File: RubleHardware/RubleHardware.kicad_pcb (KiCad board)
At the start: 4 copper layers, 56.5 x 75.4 mm, 46 parts, among them IC1 LTC3780EUH#PBF, J1_IN1 Conn_01x08_Male, J2_OUT1 Conn_01x08_Male

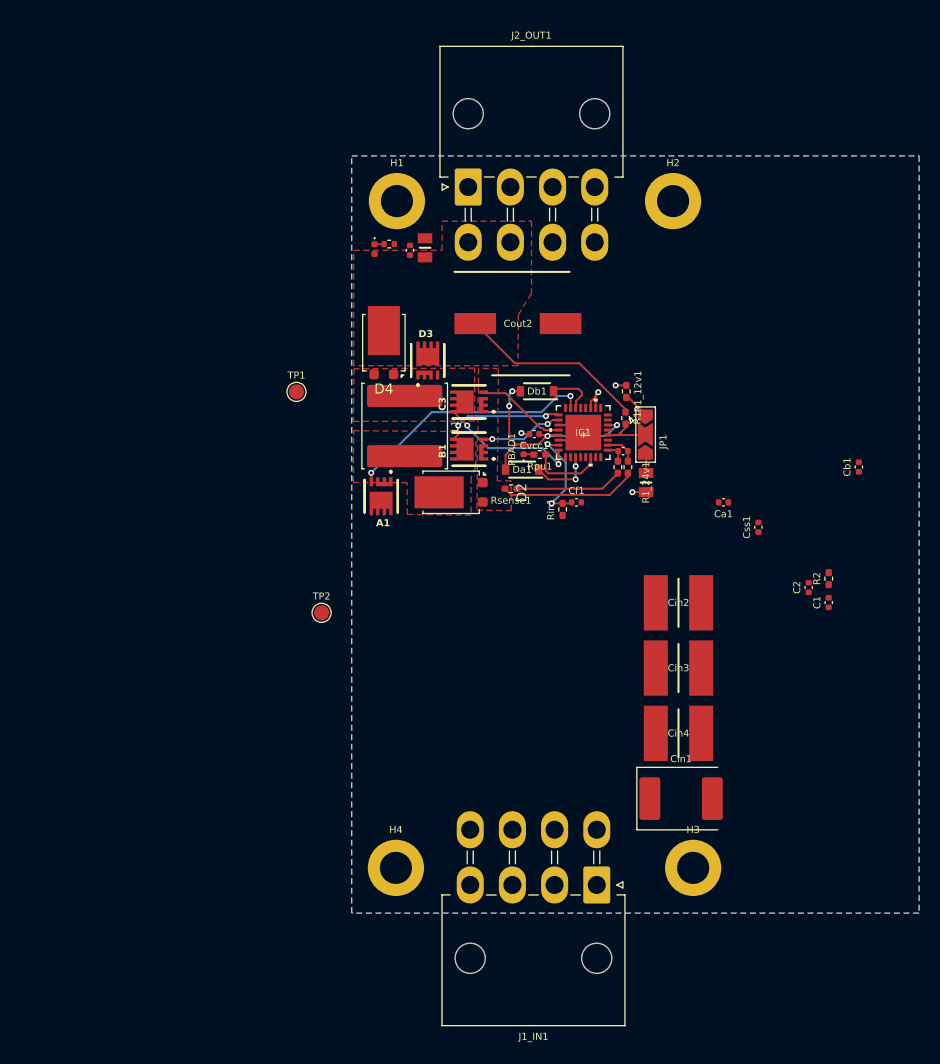
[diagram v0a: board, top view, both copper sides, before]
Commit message: feat: First board revision
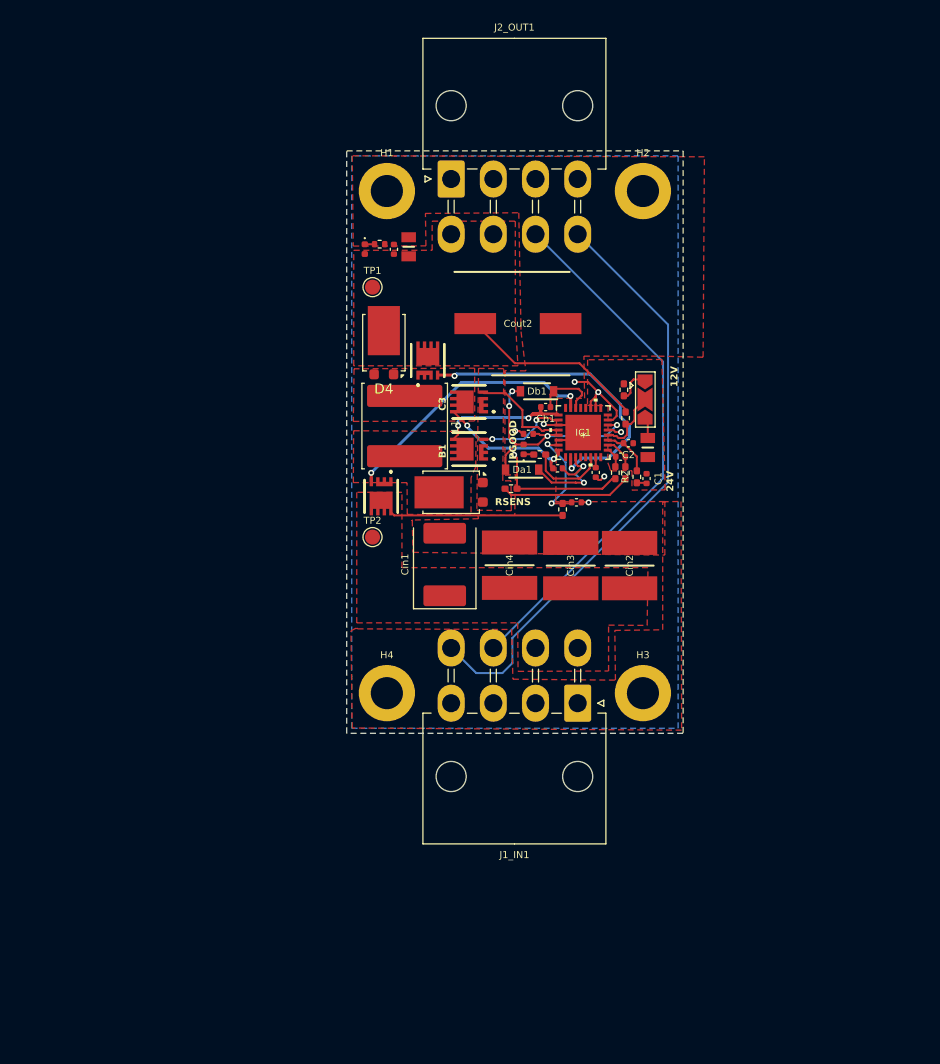
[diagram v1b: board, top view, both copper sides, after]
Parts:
- moved Cin1 33.1 mm to (168.3, 100.2), turned to 90 degrees
- moved Cb1 31.8 mm to (178.3, 84.5), turned to 180 degrees
- moved Cin4 23.7 mm to (174.7, 100.3), turned to -90 degrees
- moved C2 23.0 mm to (186.6, 88.1), turned to 180 degrees
- moved C1 21.9 mm to (188.4, 91.6), turned to -90 degrees
- moved R2 21.6 mm to (187.4, 91.5)
- moved J1_IN1 18.2 mm to (181.5, 114.0)
- moved H3 18.1 mm to (188.0, 113.0)
- moved H4 17.4 mm to (162.5, 113.0)
- moved Css1 17.1 mm to (183.3, 91.0)
- moved Ca1 16.9 mm to (179.5, 90.6)
- moved Cin3 14.8 mm to (180.8, 100.3), turned to -90 degrees
- moved TP1 12.9 mm to (161.1, 72.6)
- moved TP2 9.09 mm to (161.1, 97.5)
- moved Cin2 6.12 mm to (186.7, 100.3), turned to -90 degrees
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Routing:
- net /CAN+: track 0.00 -> 60.4 mm
- net /CAN-: track 0.00 -> 53.5 mm
- net /TG1: track 0.00 -> 31.4 mm, vias 0 -> 2
- net /ICVIN: track 0.00 -> 17.2 mm
- net GND: track 22.5 -> 34.9 mm, vias 4 -> 8
- net Net-(Da1-K): track 6.29 -> 11.8 mm
- net Net-(IC1-ITH): track 0.00 -> 5.00 mm
- net /SW2: track 12.1 -> 14.1 mm
- net Net-(Db1-K): track 4.61 -> 6.31 mm
- net /TG2: track 25.1 -> 26.2 mm
- net /BG1: track 8.99 -> 10.1 mm
- net Net-(IC1-SS): track 0.00 -> 1.07 mm
- net Net-(C1-Pad2): track 0.00 -> 0.99 mm
- net Net-(JP1-A): track 2.61 -> 3.40 mm
- net Net-(IC1-PGOOD): track 7.25 -> 7.94 mm
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- added copper zone on In2.Cu, net +3V3
- added copper zone on F.Cu, net /ICVIN
- added copper zone on B.Cu, net GND
- added copper zone on F.Cu, net GND
- added copper zone on In1.Cu, net GND
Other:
- board size 56.5 x 75.4 mm -> 33.5 x 58 mm
- board text added: "12V"
- board text added: "24V"
- board text added: "PGOOD"
- board text added: "RSENS"

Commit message: feat: Board V2
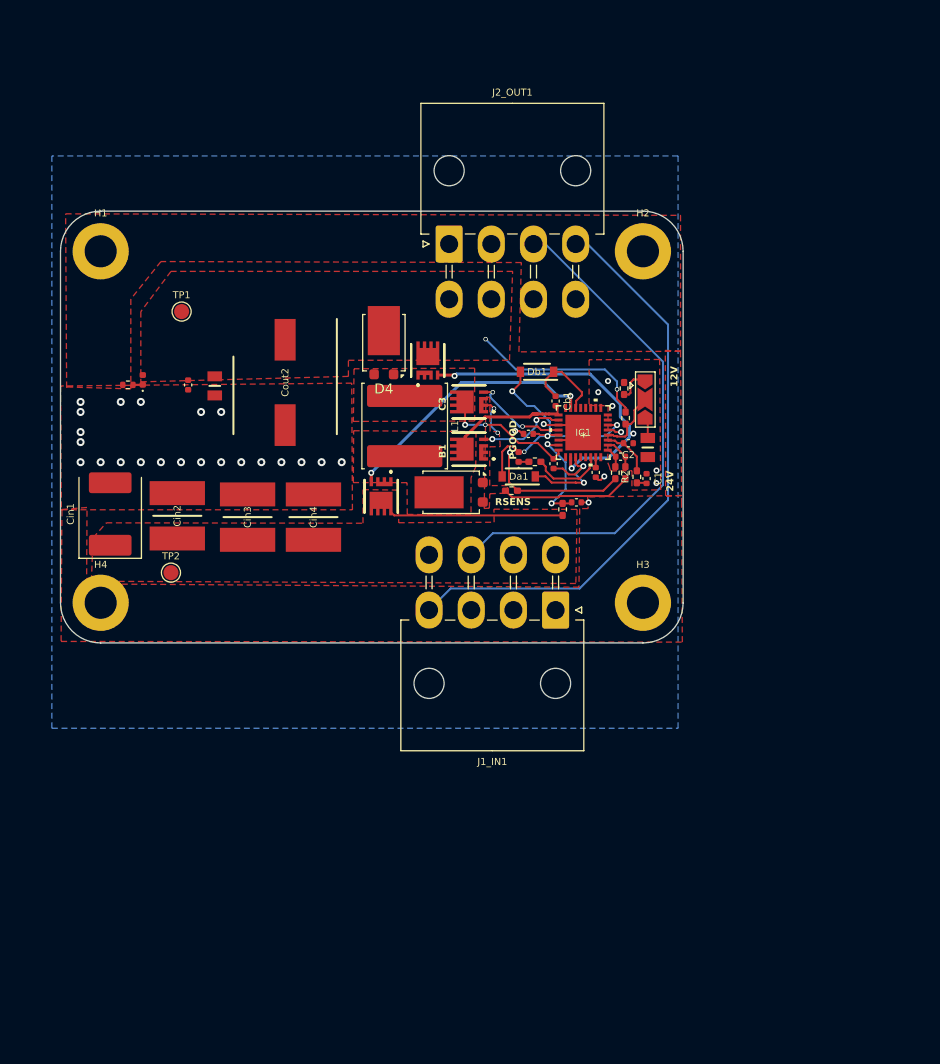
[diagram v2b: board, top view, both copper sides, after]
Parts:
- moved Cin2 45.3 mm to (141.6, 95.3)
- moved Cin1 33.7 mm to (134.9, 95.2)
- moved Cin3 32.5 mm to (148.6, 95.5)
- moved H4 29.9 mm to (134.0, 104.0)
- moved H1 29.1 mm to (134.0, 69.0)
- moved R3 28.7 mm to (136.7, 82.3), turned to 180 degrees
- moved D1 25.7 mm to (138.2, 81.8), turned to 90 degrees
- moved Cout1 24.5 mm to (142.7, 82.3), turned to -90 degrees
- moved Cout2 23.9 mm to (152.4, 82.1), turned to -90 degrees
- moved Cout3 23.8 mm to (145.4, 82.4), turned to -90 degrees
- moved TP2 20.4 mm to (141.0, 101.0)
- moved Cin4 20.1 mm to (155.2, 95.5)
- moved TP1 19.2 mm to (142.1, 75.0)
- moved J1_IN1 9.53 mm to (179.3, 104.7)
- moved H3 9.00 mm to (188.0, 104.0)
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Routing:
- net +3V3: track 0.00 -> 58.5 mm
- net /CAN-: track 53.5 -> 91.0 mm
- net /CAN+: track 60.4 -> 31.5 mm
- net GND: track 34.9 -> 25.7 mm, vias 8 -> 34
- net /INTVCC: track 26.1 -> 30.0 mm
- net /SENS-: track 13.4 -> 17.2 mm, vias 0 -> 2
- net Net-(Db1-K): track 6.31 -> 8.37 mm
- net /SW2: track 14.1 -> 13.1 mm, vias 2 -> 0
- net Net-(Da1-K): track 11.8 -> 12.5 mm
- net /ICVOUT: track 18.8 -> 18.2 mm, vias 0 -> 2
- net Net-(IC1-PGOOD): track 7.94 -> 7.42 mm
- net /BG1: track 10.1 -> 9.68 mm, vias 0 -> 2
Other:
- board size 33.5 x 58 mm -> 62 x 43 mm

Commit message: feat: v3 almost complete
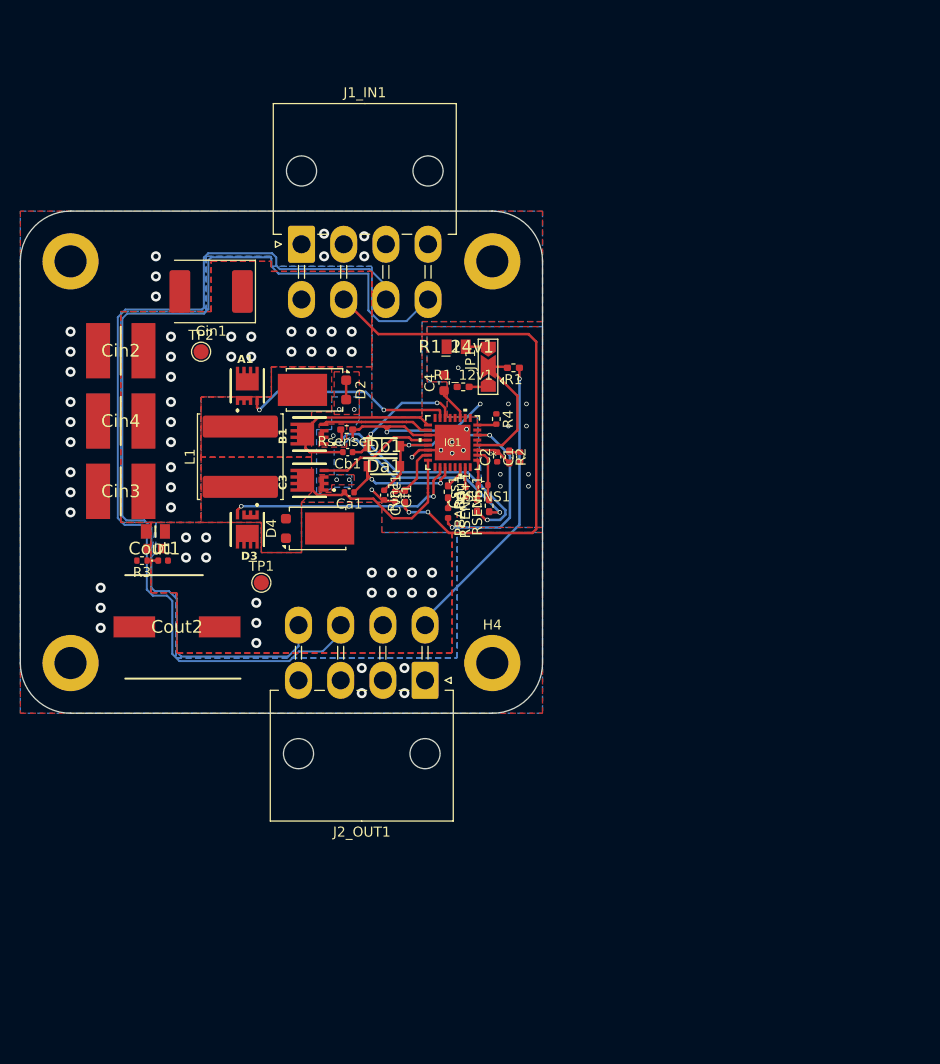
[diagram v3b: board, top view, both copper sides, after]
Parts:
- added C4: 100nF, Capacitor_SMD:C_0603_1608Metric, F.Cu at (168.2, 82.1)
- added R4: 10k, Resistor_SMD:R_0402_1005Metric, F.Cu at (173.4, 85.7)
- Ca1: value 0.22uF -> 1uF
- Cb1: value 0.22u -> 1uF
- Cout1: footprint Capacitor_SMD:C_0402_1005Metric -> iclr:CAPC1608X90N
- moved H2 70.2 mm to (131.0, 110.0)
- moved J1_IN1 44.3 mm to (154.0, 68.3), turned to 0 degrees
- moved J2_OUT1 43.5 mm to (166.3, 111.7), turned to 180 degrees
- moved H4 39.5 mm to (173.0, 110.0)
- moved H3 37.2 mm to (173.0, 70.0)
- moved TP1 28.1 mm to (150.0, 102.0)
- moved Cout2 26.6 mm to (141.6, 106.4), turned to 180 degrees
- moved D3 24.6 mm to (148.6, 96.7), turned to 180 degrees
- moved Cin1 24.3 mm to (145.0, 73.0), turned to 180 degrees
- moved TP2 22.2 mm to (144.0, 79.0)
- moved R1_24v1 21.6 mm to (169.4, 78.5), turned to 0 degrees
- moved Cin4 21.4 mm to (136.0, 85.9), turned to 0 degrees
- moved Cb1 21.3 mm to (158.6, 89.0), turned to 180 degrees
- moved Ca1 20.5 mm to (158.8, 93.0), turned to 180 degrees
- moved D4 19.6 mm to (155.6, 96.6), turned to 90 degrees
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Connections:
- B1 pad 1: /SENS- -> /SENS+
- B1 pad 2: /SENS- -> /SENS+
- B1 pad 3: /SENS- -> /SENS+
- B1 pad A1: /SENS- -> /SENS+
- C3 pad 1: /SENS- -> /SENS+
- C3 pad 2: /SENS- -> /SENS+
- C3 pad 3: /SENS- -> /SENS+
- C3 pad A1: /SENS- -> /SENS+
- D2 pad 1: /SENS- -> /SENS+
- D2 pad 2: /SENS- -> /SENS+
- IC1 pad 11: GND -> Net-(IC1-STBYMD)
- IC1 pad 8: unconnected-(IC1-PLLFTR-Pad8) -> Net-(IC1-PLLFTR)
- RSENS+1 pad 1: GND -> /SENS+
- RSENS-1 pad 1: /SENS- -> GND
- Rsense1 pad 2: /SENS- -> /SENS+
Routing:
- net /CAN+: track 31.5 -> 95.4 mm
- net +3V3: track 58.5 -> 0.00 mm
- net /ICVIN: track 17.2 -> 54.5 mm, vias 0 -> 23
- net /SENS+: track 0.00 -> 27.3 mm, vias 0 -> 7
- net GND: track 25.7 -> 49.7 mm, vias 34 -> 44
- net /SENS-: track 17.2 -> 0.00 mm, vias 2 -> 0
- net /ICVOUT: track 18.2 -> 29.5 mm, vias 2 -> 16
- net /TG1: track 31.4 -> 23.8 mm
- net Net-(IC1-VOSENSE): track 6.79 -> 14.1 mm
- net /SW2: track 13.1 -> 18.7 mm
- net /SW1: track 13.6 -> 19.0 mm, vias 2 -> 0
- net Net-(IC1-PGOOD): track 7.42 -> 2.35 mm
- net /TG2: track 26.2 -> 21.3 mm
- net Net-(IC1-VIN): track 10.4 -> 5.80 mm, vias 2 -> 0
- net Net-(Db1-K): track 8.37 -> 13.0 mm, vias 0 -> 2
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- added copper zone on B.Cu, net /ICVIN
- added copper zone on B.Cu, net /ICVOUT
- added copper zone on B.Cu, net /SENS+
- added copper zone on F.Cu, net /SENS+
- removed copper zone on F.Cu, net /SENS-
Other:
- board size 62 x 43 mm -> 52 x 50 mm
- board text removed: "12V"
- board text removed: "24V"
- board text removed: "PGOOD"
- board text removed: "PWR"
- board text removed: "RSENS"
